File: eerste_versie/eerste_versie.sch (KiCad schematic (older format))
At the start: 13 parts, among them U1 ESP32-WROOM-32U, U2 AMS1117-3.3, X1 DG3XX-02-5.0

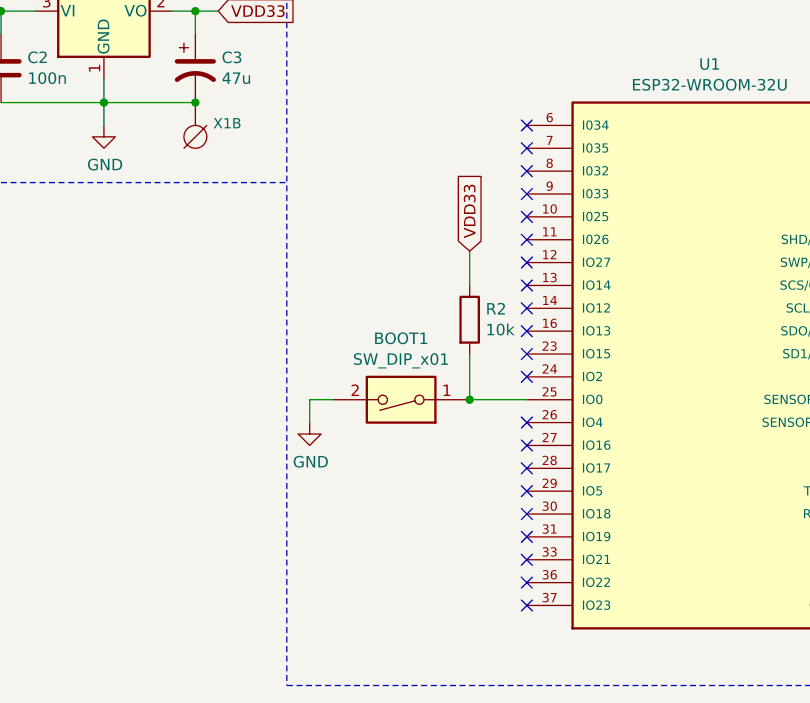
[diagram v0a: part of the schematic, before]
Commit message: update
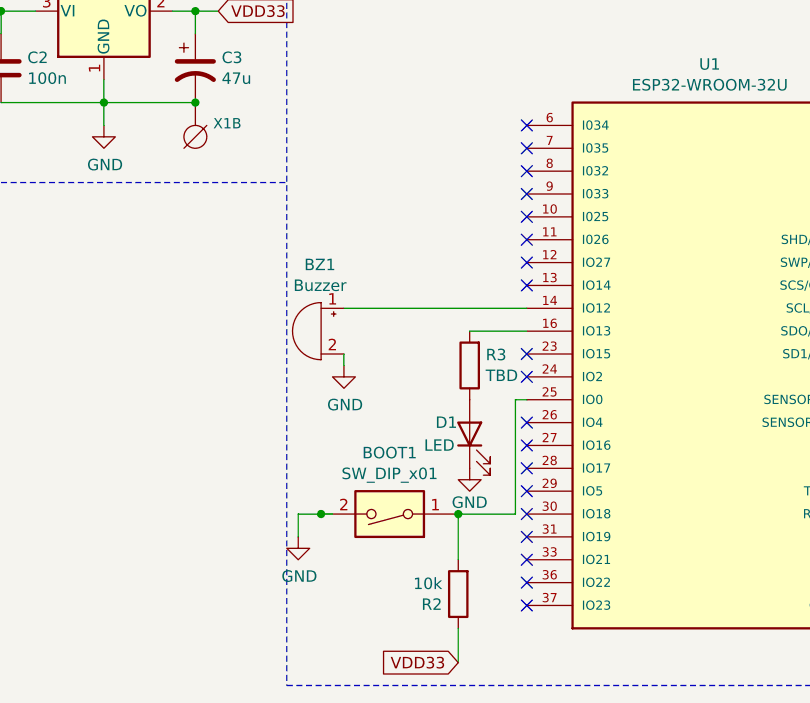
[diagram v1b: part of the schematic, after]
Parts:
- added BZ1: Buzzer, CPT-1255C-090:CUI_CPT-1255C-090, symbol Device:Buzzer
- added D1: LED, LED_SMD:LED_0805_2012Metric_Pad1.15x1.40mm_HandSolder, symbol Device:LED
- added R3: TBD, Resistor_SMD:R_0805_2012Metric_Pad1.20x1.40mm_HandSolder, symbol Device:R
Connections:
- net GND: now also BZ1.2 (+), D1.1 (K)
- net at U1.14 (IO12): now also BZ1.1 (-)
- net at U1.16 (IO13): now also R3.2
- new net: D1.2 (A), R3.1
- no-connect marks 29 -> 27
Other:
- moved on the sheet: BOOT1, R2
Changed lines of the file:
@@
 	1    0    0    -1
-$EndComp
-Wire Wire Line
-	2850 2900 2850 3000
-Wire Wire Line
-	2950 2900 2850 2900
-$Comp
-L power:GND #PWR04
-U 1 1 60453368
-P 2850 3000
-F 0 "#PWR04" H 2850 2750 50  0001 C CNN
-F 1 "GND" H 2855 2827 50  0000 C CNN
-F 2 "" H 2850 3000 50  0001 C CNN
-F 3 "" H 2850 3000 50  0001 C CNN
-	1    2850 3000
-	1    0    0    -1
-$EndComp
-$Comp
-L Switch:SW_DIP_x01 BOOT1
-U 1 1 60452495
-P 3250 2900
-F 0 "BOOT1" H 3250 2633 50  0000 C CNN
-F 1 "SW_DIP_x01" H 3250 2724 50  0000 C CNN
-F 2 "Button_Switch_SMD:SW_SPST_B3U-1000P" H 3250 2900 50  0001 C CNN
-F 3 "~" H 3250 2900 50  0001 C CNN
-	1    3250 2900
-	-1   0    0    1
 $EndComp
 Connection ~ 5400 1400
@@
 NoConn ~ 3800 2800
 NoConn ~ 3800 2700
-NoConn ~ 3800 2600
-NoConn ~ 3800 2500
 NoConn ~ 3800 2400
 NoConn ~ 3800 2300
@@
 Text Notes 3050 750  0    79   ~ 0
 ESP32
+Wire Wire Line
+	2800 3400 2800 3500
+Wire Wire Line
+	2900 3400 2800 3400
+$Comp
+L power:GND #PWR04
+U 1 1 60453368
+P 2800 3500
+F 0 "#PWR04" H 2800 3250 50  0001 C CNN
+F 1 "GND" H 2805 3327 50  0000 C CNN
+F 2 "" H 2800 3500 50  0001 C CNN
+F 3 "" H 2800 3500 50  0001 C CNN
+	1    2800 3500
+	1    0    0    -1
+$EndComp
 $Comp
 L Device:R R2
 U 1 1 60511A7D
-P 3550 2550
-F 0 "R2" H 3620 2596 50  0000 L CNN
-F 1 "10k" H 3620 2505 50  0000 L CNN
-F 2 "Resistor_SMD:R_0805_2012Metric_Pad1.20x1.40mm_HandSolder" V 3480 2550 50  0001 C CNN
-F 3 "~" H 3550 2550 50  0001 C CNN
-	1    3550 2550
-	1    0    0    -1
-$EndComp
-Wire Wire Line
-	3550 2700 3550 2900
-Text GLabel 3550 2250 1    50   Input ~ 0
+P 3500 3750
+F 0 "R2" H 3570 3796 50  0000 L CNN
+F 1 "10k" H 3570 3705 50  0000 L CNN
+F 2 "Resistor_SMD:R_0805_2012Metric_Pad1.20x1.40mm_HandSolder" V 3430 3750 50  0001 C CNN
+F 3 "~" H 3500 3750 50  0001 C CNN
+	1    3500 3750
+	-1   0    0    1
+$EndComp
+Wire Wire Line
+	3500 3600 3500 3400
+Text GLabel 3500 4050 0    50   Input ~ 0
 VDD33
 Wire Wire Line
-	3550 2250 3550 2400
-Wire Wire Line
-	3550 2900 3800 2900
-Connection ~ 3550 2900
+	3500 4050 3500 3900
+Wire Wire Line
+	3500 3400 3750 3400
+Connection ~ 3500 3400
+$Comp
+L Switch:SW_DIP_x01 BOOT1
+U 1 1 60452495
+P 3200 3400
+F 0 "BOOT1" H 3200 3133 50  0000 C CNN
+F 1 "SW_DIP_x01" H 3200 3224 50  0000 C CNN
+F 2 "Button_Switch_SMD:SW_SPST_B3U-1000P" H 3200 3400 50  0001 C CNN
+F 3 "~" H 3200 3400 50  0001 C CNN
+	1    3200 3400
+	-1   0    0    1
+$EndComp
+$Comp
+L Device:Buzzer BZ1
+U 1 1 6052D7F8
+P 2900 2600
+F 0 "BZ1" H 2905 2890 50  0000 C CNN
+F 1 "Buzzer" H 2905 2799 50  0000 C CNN
+F 2 "CPT-1255C-090:CUI_CPT-1255C-090" V 2875 2700 50  0001 C CNN
+F 3 "~" V 2875 2700 50  0001 C CNN
+	1    2900 2600
+	-1   0    0    -1
+$EndComp
+Wire Wire Line
+	3000 2500 3800 2500
+Wire Wire Line
+	2950 3400 2900 3400
+Connection ~ 2900 3400
+$Comp
+L Device:R R3
+U 1 1 6053C92B
+P 3550 2750
+F 0 "R3" H 3480 2704 50  0000 R CNN
+F 1 "TBD" H 3480 2795 50  0000 R CNN
+F 2 "Resistor_SMD:R_0805_2012Metric_Pad1.20x1.40mm_HandSolder" V 3480 2750 50  0001 C CNN
+F 3 "~" H 3550 2750 50  0001 C CNN
+	1    3550 2750
+	-1   0    0    1
+$EndComp
+$Comp
+L Device:LED D1
+U 1 1 6053D592
+P 3550 3050
+F 0 "D1" V 3600 3200 50  0000 R CNN
+F 1 "LED" V 3500 3250 50  0000 R CNN
+F 2 "LED_SMD:LED_0805_2012Metric_Pad1.15x1.40mm_HandSolder" H 3550 3050 50  0001 C CNN
+F 3 "~" H 3550 3050 50  0001 C CNN
+	1    3550 3050
+	0    -1   -1   0
+$EndComp
+Wire Wire Line
+	3800 2600 3550 2600
+$Comp
+L power:GND #PWR09
+U 1 1 6053EC09
+P 3550 3200
+F 0 "#PWR09" H 3550 2950 50  0001 C CNN
+F 1 "GND" H 3550 3050 50  0000 C CNN
+F 2 "" H 3550 3200 50  0001 C CNN
+F 3 "" H 3550 3200 50  0001 C CNN
+	1    3550 3200
+	1    0    0    -1
+$EndComp
+Wire Wire Line
+	3800 2900 3750 2900
+Wire Wire Line
+	3750 2900 3750 3400
+$Comp
+L power:GND #PWR08
+U 1 1 60540F03
+P 3000 2750
+F 0 "#PWR08" H 3000 2500 50  0001 C CNN
+F 1 "GND" H 3005 2577 50  0000 C CNN
+F 2 "" H 3000 2750 50  0001 C CNN
+F 3 "" H 3000 2750 50  0001 C CNN
+	1    3000 2750
+	1    0    0    -1
+$EndComp
+Wire Wire Line
+	3000 2700 3000 2750
 $EndSCHEMATC
